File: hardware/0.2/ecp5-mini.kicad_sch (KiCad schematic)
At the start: 28 parts, among them J3 S7 Mini, J4 S7 Mini, U2 ECP5U_12_CABGA256, X1 16MHz

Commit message: bom fix
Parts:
- C1, C504, C505, C510, C511, C514, C520: MPN CC0402KRX7R7BB103 -> CC0402KRX7R7BB104
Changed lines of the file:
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@@
     (company "Josh Johnson")
   )
+  (bus_alias "LED" (members "LED_[0..7]" "LED_R" "LED_G" "LED_B"))
+  (bus_alias "HYPERRAM" (members "HR_nRST" "HR_nCS" "HR_CK_N" "HR_RWDS" "HR_DQ[0..7]" "HR_CK_P" "HR_nCK"))
+  (bus_alias "USB" (members "USB_D-" "USB_D+" "USB_PU"))
   (bus_alias "SD" (members "SD_DAT[0..3]" "SD_CMD" "SD_CLK" "SD_DET"))
-  (bus_alias "USB" (members "USB_D-" "USB_D+" "USB_PU"))
-  (bus_alias "HYPERRAM" (members "HR_nRST" "HR_nCS" "HR_CK_N" "HR_RWDS" "HR_DQ[0..7]" "HR_CK_P" "HR_nCK"))
-  (bus_alias "LED" (members "LED_[0..7]" "LED_R" "LED_G" "LED_B"))
   (junction (at 60.96 58.42) (diameter 1.016) (color 0 0 0 0))
   (junction (at 62.23 176.53) (diameter 1.016) (color 0 0 0 0))
@@
   (junction (at 358.14 196.85) (diameter 1.016) (color 0 0 0 0))
   (junction (at 358.14 198.12) (diameter 1.016) (color 0 0 0 0))
-  (no_connect (at 50.8 116.84))
-  (no_connect (at 50.8 215.9))
-  (no_connect (at 138.43 242.57))
-  (no_connect (at 137.16 106.68))
-  (no_connect (at 218.44 86.36))
-  (no_connect (at 138.43 219.71))
-  (no_connect (at 50.8 198.12))
+  (no_connect (at 215.9 238.76))
+  (no_connect (at 50.8 109.22))
+  (no_connect (at 50.8 238.76))
+  (no_connect (at 138.43 240.03))
   (no_connect (at 137.16 149.86))
-  (no_connect (at 50.8 259.08))
-  (no_connect (at 215.9 215.9))
-  (no_connect (at 215.9 220.98))
-  (no_connect (at 215.9 236.22))
-  (no_connect (at 215.9 269.24))
-  (no_connect (at 50.8 213.36))
-  (no_connect (at 137.16 154.94))
-  (no_connect (at 215.9 200.66))
-  (no_connect (at 50.8 106.68))
-  (no_connect (at 218.44 160.02))
-  (no_connect (at 137.16 116.84))
-  (no_connect (at 50.8 132.08))
-  (no_connect (at 215.9 208.28))
-  (no_connect (at 50.8 274.32))
-  (no_connect (at 138.43 250.19))
-  (no_connect (at 218.44 129.54))
-  (no_connect (at 137.16 88.9))
-  (no_connect (at 137.16 121.92))
-  (no_connect (at 215.9 246.38))
-  (no_connect (at 50.8 210.82))
-  (no_connect (at 215.9 238.76))
-  (no_connect (at 215.9 218.44))
-  (no_connect (at 50.8 129.54))
-  (no_connect (at 50.8 233.68))
-  (no_connect (at 138.43 270.51))
-  (no_connect (at 50.8 121.92))
-  (no_connect (at 215.9 271.78))
-  (no_connect (at 215.9 266.7))
-  (no_connect (at 137.16 119.38))
-  (no_connect (at 138.43 240.03))
-  (no_connect (at 50.8 266.7))
-  (no_connect (at 138.43 262.89))
-  (no_connect (at 50.8 251.46))
-  (no_connect (at 50.8 271.78))
   (no_connect (at 218.44 96.52))
-  (no_connect (at 218.44 109.22))
-  (no_connect (at 218.44 137.16))
-  (no_connect (at 218.44 157.48))
-  (no_connect (at 50.8 203.2))
-  (no_connect (at 138.43 273.05))
-  (no_connect (at 50.8 256.54))
-  (no_connect (at 215.9 203.2))
-  (no_connect (at 137.16 86.36))
-  (no_connect (at 218.44 106.68))
-  (no_connect (at 50.8 238.76))
-  (no_connect (at 50.8 127))
-  (no_connect (at 215.9 205.74))
-  (no_connect (at 218.44 147.32))
-  (no_connect (at 218.44 88.9))
   (no_connect (at 50.8 228.6))
   (no_connect (at 218.44 99.06))
+  (no_connect (at 215.9 205.74))
+  (no_connect (at 218.44 160.02))
+  (no_connect (at 215.9 220.98))
+  (no_connect (at 50.8 119.38))
+  (no_connect (at 50.8 91.44))
+  (no_connect (at 138.43 260.35))
+  (no_connect (at 215.9 266.7))
+  (no_connect (at 215.9 203.2))
+  (no_connect (at 138.43 222.25))
+  (no_connect (at 50.8 274.32))
+  (no_connect (at 50.8 198.12))
+  (no_connect (at 218.44 149.86))
+  (no_connect (at 218.44 127))
+  (no_connect (at 50.8 213.36))
+  (no_connect (at 138.43 217.17))
+  (no_connect (at 138.43 270.51))
+  (no_connect (at 50.8 251.46))
+  (no_connect (at 137.16 119.38))
+  (no_connect (at 218.44 88.9))
+  (no_connect (at 215.9 200.66))
+  (no_connect (at 50.8 259.08))
+  (no_connect (at 138.43 262.89))
+  (no_connect (at 218.44 147.32))
+  (no_connect (at 138.43 242.57))
+  (no_connect (at 137.16 109.22))
+  (no_connect (at 137.16 106.68))
+  (no_connect (at 50.8 127))
+  (no_connect (at 138.43 252.73))
+  (no_connect (at 50.8 104.14))
+  (no_connect (at 50.8 101.6))
   (no_connect (at 137.16 99.06))
-  (no_connect (at 138.43 222.25))
+  (no_connect (at 218.44 86.36))
+  (no_connect (at 137.16 124.46))
+  (no_connect (at 218.44 106.68))
+  (no_connect (at 215.9 218.44))
+  (no_connect (at 215.9 208.28))
+  (no_connect (at 50.8 203.2))
+  (no_connect (at 137.16 121.92))
+  (no_connect (at 50.8 215.9))
+  (no_connect (at 50.8 116.84))
+  (no_connect (at 50.8 210.82))
   (no_connect (at 137.16 157.48))
+  (no_connect (at 50.8 233.68))
+  (no_connect (at 215.9 261.62))
+  (no_connect (at 50.8 236.22))
+  (no_connect (at 218.44 137.16))
+  (no_connect (at 137.16 154.94))
+  (no_connect (at 138.43 273.05))
+  (no_connect (at 218.44 129.54))
+  (no_connect (at 138.43 214.63))
+  (no_connect (at 50.8 106.68))
+  (no_connect (at 215.9 246.38))
+  (no_connect (at 215.9 269.24))
+  (no_connect (at 137.16 86.36))
+  (no_connect (at 218.44 139.7))
+  (no_connect (at 50.8 132.08))
+  (no_connect (at 50.8 129.54))
+  (no_connect (at 215.9 223.52))
+  (no_connect (at 137.16 116.84))
+  (no_connect (at 50.8 269.24))
+  (no_connect (at 138.43 219.71))
+  (no_connect (at 215.9 271.78))
+  (no_connect (at 218.44 157.48))
+  (no_connect (at 215.9 236.22))
+  (no_connect (at 50.8 256.54))
+  (no_connect (at 50.8 121.92))
+  (no_connect (at 138.43 250.19))
+  (no_connect (at 137.16 96.52))
+  (no_connect (at 137.16 160.02))
+  (no_connect (at 50.8 266.7))
+  (no_connect (at 137.16 88.9))
+  (no_connect (at 50.8 271.78))
+  (no_connect (at 215.9 215.9))
   (no_connect (at 50.8 254))
-  (no_connect (at 50.8 119.38))
-  (no_connect (at 137.16 109.22))
-  (no_connect (at 215.9 223.52))
-  (no_connect (at 50.8 101.6))
-  (no_connect (at 218.44 149.86))
-  (no_connect (at 50.8 269.24))
-  (no_connect (at 138.43 260.35))
-  (no_connect (at 137.16 160.02))
-  (no_connect (at 50.8 109.22))
-  (no_connect (at 50.8 91.44))
-  (no_connect (at 218.44 139.7))
-  (no_connect (at 138.43 214.63))
-  (no_connect (at 137.16 96.52))
-  (no_connect (at 215.9 261.62))
-  (no_connect (at 137.16 124.46))
-  (no_connect (at 138.43 217.17))
-  (no_connect (at 218.44 127))
-  (no_connect (at 50.8 104.14))
-  (no_connect (at 50.8 236.22))
-  (no_connect (at 138.43 252.73))
+  (no_connect (at 218.44 109.22))
   (bus_entry (at 62.23 81.28) (size 2.54 -2.54)
     (stroke (width 0.1524) (type solid) (color 0 0 0 0))
@@
       (effects (font (size 1.27 1.27)) hide)
     )
-    (property "MPN" "CC0402KRX7R7BB103" (id 5) (at 60.96 63.5 0)
+    (property "MPN" "CC0402KRX7R7BB104" (id 5) (at 60.96 63.5 0)
       (effects (font (size 1.27 1.27)) hide)
     )
@@
       (effects (font (size 1.27 1.27)) hide)
     )
-    (property "MPN" "CC0402KRX7R7BB103" (id 5) (at 62.23 181.61 0)
+    (property "MPN" "CC0402KRX7R7BB104" (id 5) (at 62.23 181.61 0)
       (effects (font (size 1.27 1.27)) hide)
     )
@@
       (effects (font (size 1.27 1.27)) hide)
     )
-    (property "MPN" "CC0402KRX7R7BB103" (id 5) (at 148.59 67.31 0)
+    (property "MPN" "CC0402KRX7R7BB104" (id 5) (at 148.59 67.31 0)
       (effects (font (size 1.27 1.27)) hide)
     )
@@
       (effects (font (size 1.27 1.27)) hide)
     )
-    (property "MPN" "CC0402KRX7R7BB103" (id 5) (at 156.21 181.61 0)
+    (property "MPN" "CC0402KRX7R7BB104" (id 5) (at 156.21 181.61 0)
       (effects (font (size 1.27 1.27)) hide)
     )
@@
       (effects (font (size 1.27 1.27)) hide)
     )
-    (property "MPN" "CC0402KRX7R7BB103" (id 5) (at 228.6 181.61 0)
+    (property "MPN" "CC0402KRX7R7BB104" (id 5) (at 228.6 181.61 0)
       (effects (font (size 1.27 1.27)) hide)
     )
@@
       (effects (font (size 1.27 1.27)) hide)
     )
-    (property "MPN" "CC0402KRX7R7BB103" (id 5) (at 229.87 67.31 0)
+    (property "MPN" "CC0402KRX7R7BB104" (id 5) (at 229.87 67.31 0)
       (effects (font (size 1.27 1.27)) hide)
     )
@@
       (effects (font (size 1.27 1.27)) hide)
     )
-    (property "MPN" "CC0402KRX7R7BB103" (id 5) (at 361.95 201.93 0)
-      (effects (font (size 1.27 1.27)) hide)
-    )
+    (property "MPN" "CC0402KRX7R7BB104" (id 5) (at 361.95 201.93 0)
+      (effects (font (size 1.27 1.27)) hide)
+    )

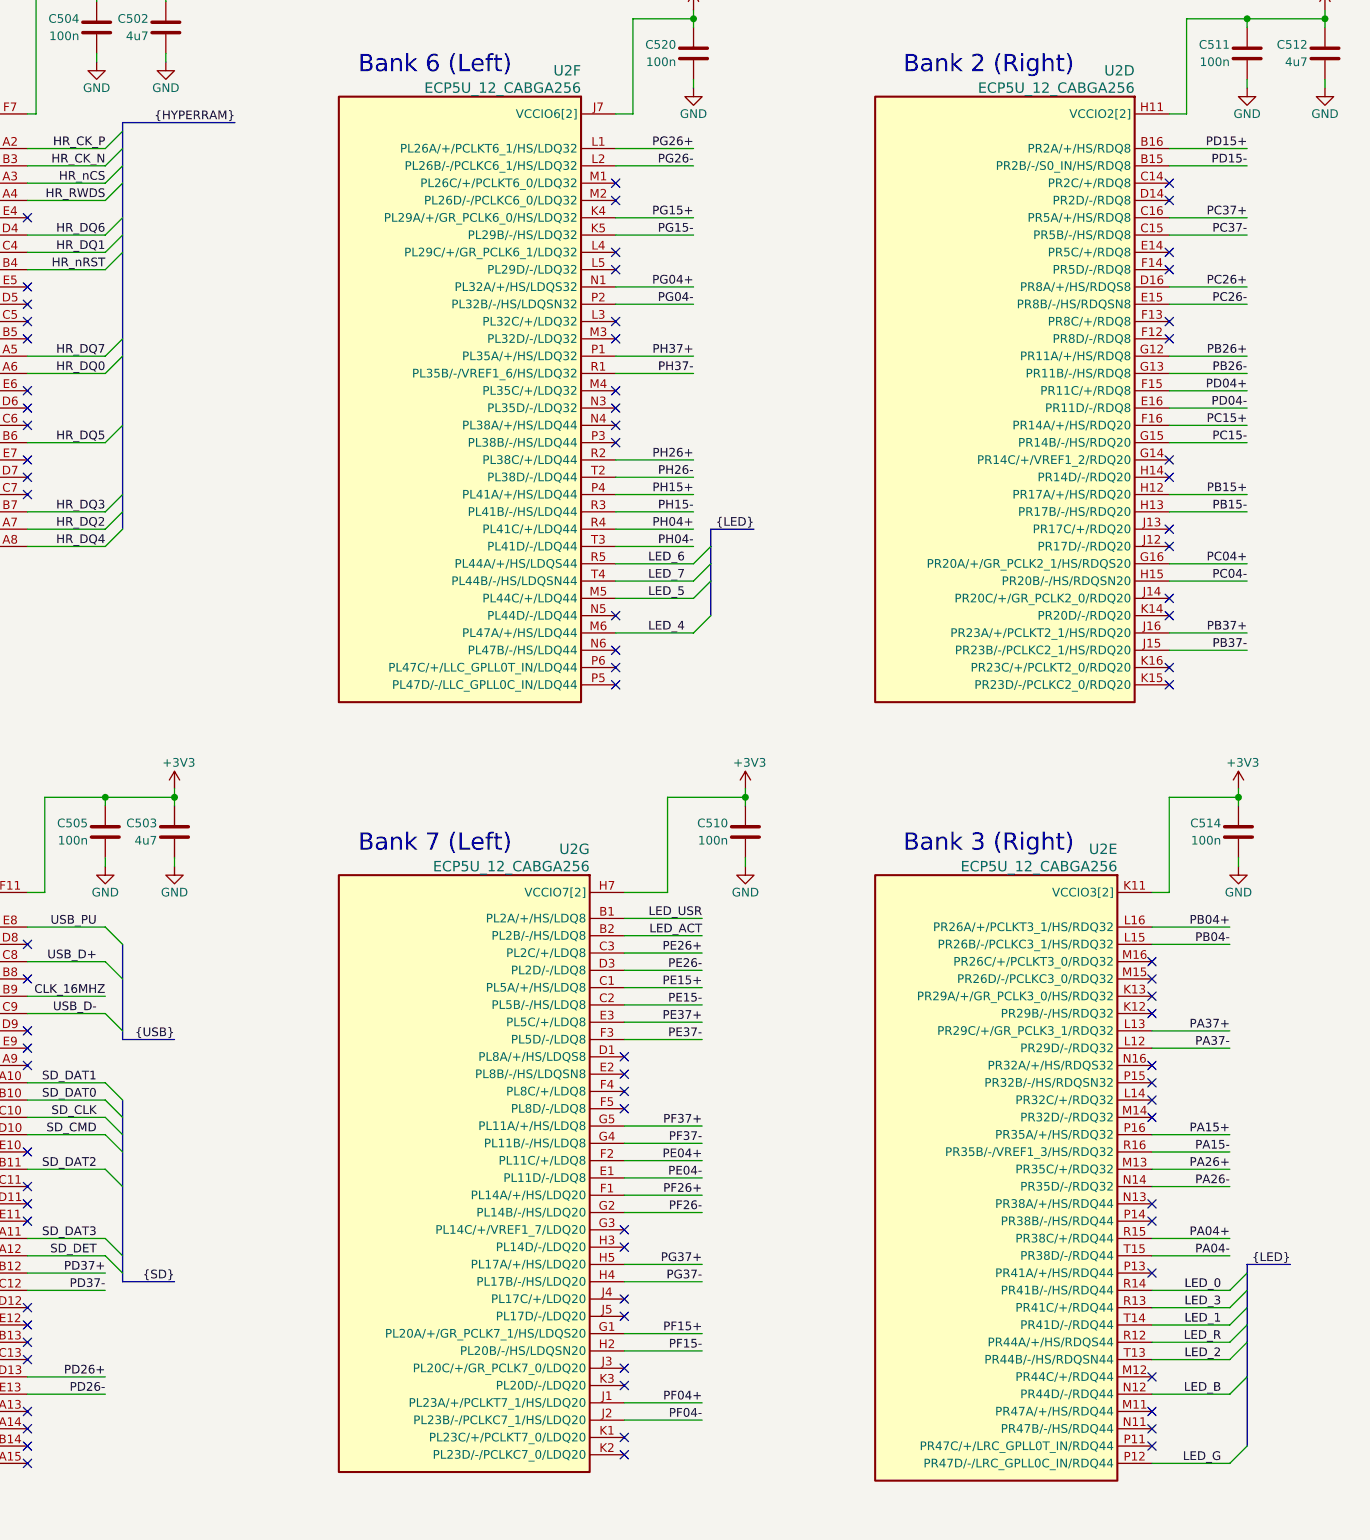
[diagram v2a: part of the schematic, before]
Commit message: nightly version bump
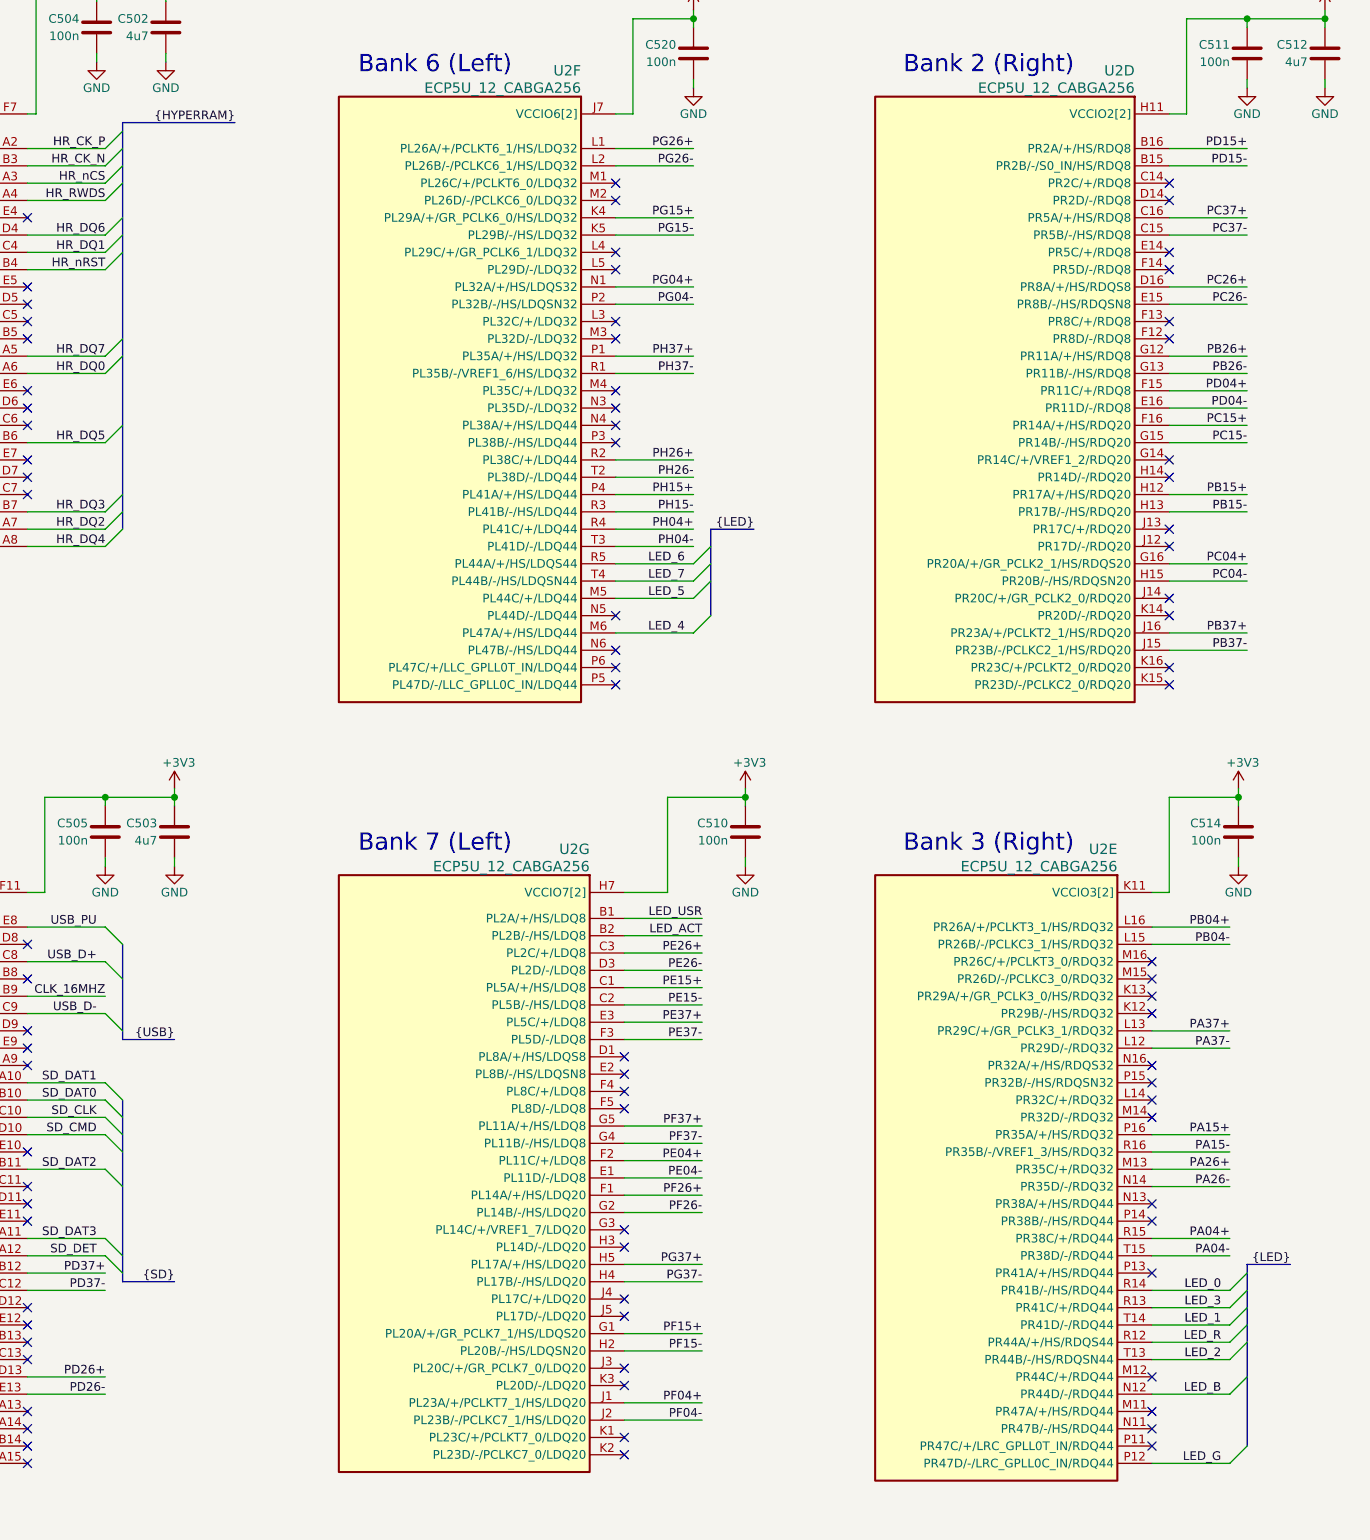
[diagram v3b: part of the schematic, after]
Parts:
- C1, C504, C505, C510, C511, C514, C520: MPN2 CL05B104KO5NNNC -> (none)
- C502, C503, C512: MPN2 CL05A475KP5NRNC -> (none)
- R500, R502, R503: MPN2 0402WGF1501TCE -> (none)
- X1: LCSC C387369 -> (none)
